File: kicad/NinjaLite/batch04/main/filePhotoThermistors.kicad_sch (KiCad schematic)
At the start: 10 parts, among them U8 TS12A12511DCNR, U9 SN74LV4051A

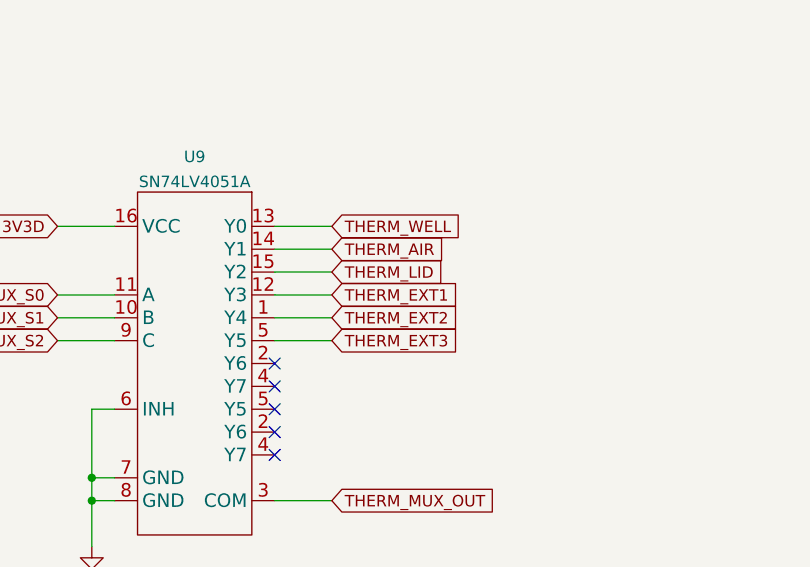
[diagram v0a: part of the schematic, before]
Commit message: wiring batch04/main
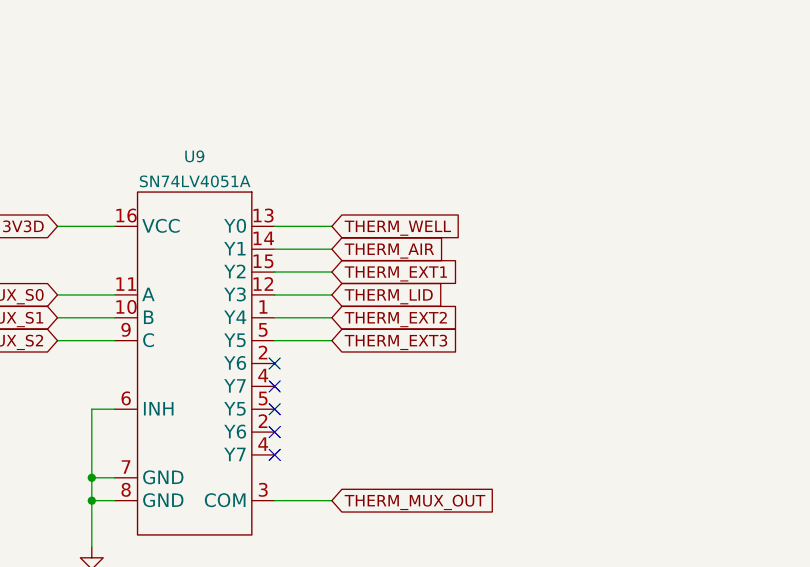
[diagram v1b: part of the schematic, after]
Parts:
- TEXT1, TEXT2, TEXT3: footprint Pin_Headers:Pin_Header_Straight_1x02_Pitch1.27mm -> Pin_Headers:Pin_Header_Straight_1x02_Pitch2.54mm
- U8: footprint Package_TO_SOT_SMD:SOT-23-8 -> Ninja-qPCR:SOT-23-8-8.3mil
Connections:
- net THERM_EXT1: now also U9.15 (Y2); no longer U9.12 (Y3)
- net THERM_LID: now also U9.12 (Y3); no longer U9.15 (Y2)
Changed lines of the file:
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@@
     )
   )
-  (global_label "THERM_LID" (shape input) (at 170.18 87.63 0) (fields_autoplaced)
-    (effects (font (size 1.27 1.27)) (justify left))
-    (property "Intersheet References" "${INTERSHEET_REFS}" (id 0) (at -25.4 36.83 0)
+  (global_label "THERM_LID" (shape input) (at 170.18 90.17 0) (fields_autoplaced)
+    (effects (font (size 1.27 1.27)) (justify left))
+    (property "Intersheet References" "${INTERSHEET_REFS}" (id 0) (at -25.4 39.37 0)
       (effects (font (size 1.27 1.27)) hide)
     )
@@
     )
   )
-  (global_label "THERM_EXT1" (shape input) (at 170.18 90.17 0) (fields_autoplaced)
-    (effects (font (size 1.27 1.27)) (justify left))
-    (property "Intersheet References" "${INTERSHEET_REFS}" (id 0) (at -25.4 31.75 0)
+  (global_label "THERM_EXT1" (shape input) (at 170.18 87.63 0) (fields_autoplaced)
+    (effects (font (size 1.27 1.27)) (justify left))
+    (property "Intersheet References" "${INTERSHEET_REFS}" (id 0) (at -25.4 29.21 0)
       (effects (font (size 1.27 1.27)) hide)
     )
@@
       (effects (font (size 1.524 1.524)))
     )
-    (property "Footprint" "Package_TO_SOT_SMD:SOT-23-8" (id 2) (at 64.77 85.344 0)
+    (property "Footprint" "Ninja-qPCR:SOT-23-8-8.3mil" (id 2) (at 64.77 85.344 0)
       (effects (font (size 1.524 1.524)) hide)
     )
@@
     (property "Reference" "TEXT1" (id 0) (at 257.81 80.01 0))
     (property "Value" "Conn_01x02_Male" (id 1) (at 264.16 82.55 0))
-    (property "Footprint" "Pin_Headers:Pin_Header_Straight_1x02_Pitch1.27mm" (id 2) (at 254 80.01 0)
+    (property "Footprint" "Pin_Headers:Pin_Header_Straight_1x02_Pitch2.54mm" (id 2) (at 254 80.01 0)
       (effects (font (size 1.27 1.27)) hide)
     )
@@
     (property "Reference" "TEXT2" (id 0) (at 257.81 88.9 0))
     (property "Value" "Conn_01x02_Male" (id 1) (at 264.16 91.44 0))
-    (property "Footprint" "Pin_Headers:Pin_Header_Straight_1x02_Pitch1.27mm" (id 2) (at 254 88.9 0)
+    (property "Footprint" "Pin_Headers:Pin_Header_Straight_1x02_Pitch2.54mm" (id 2) (at 254 88.9 0)
       (effects (font (size 1.27 1.27)) hide)
     )
@@
     (property "Reference" "TEXT3" (id 0) (at 257.81 96.52 0))
     (property "Value" "Conn_01x02_Male" (id 1) (at 264.16 99.06 0))
-    (property "Footprint" "Pin_Headers:Pin_Header_Straight_1x02_Pitch1.27mm" (id 2) (at 254 96.52 0)
-      (effects (font (size 1.27 1.27)) hide)
-    )
+    (property "Footprint" "Pin_Headers:Pin_Header_Straight_1x02_Pitch2.54mm" (id 2) (at 254 96.52 0)
+      (effects (font (size 1.27 1.27)) hide)
+    )
